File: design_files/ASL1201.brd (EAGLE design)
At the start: 12.5 x 18.5 mm, 3 parts, among them J1 LPPB051NGCN-RC, J2 S2B-PH-SM4

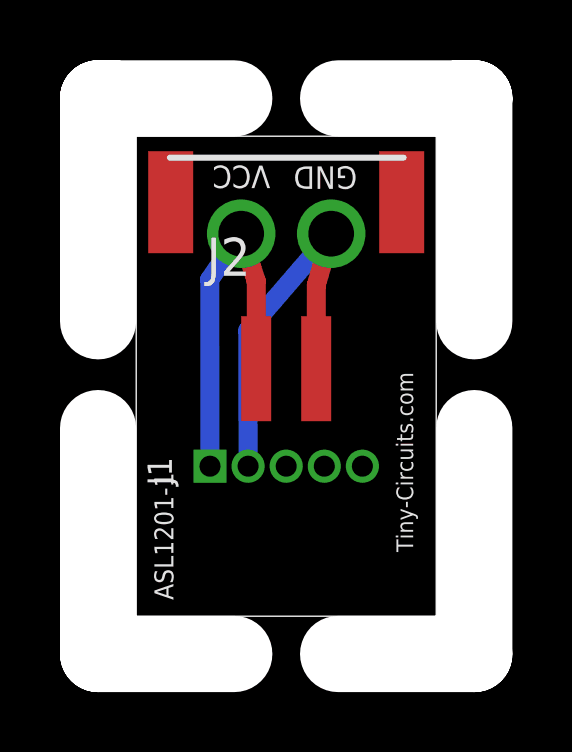
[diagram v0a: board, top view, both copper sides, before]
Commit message: update format
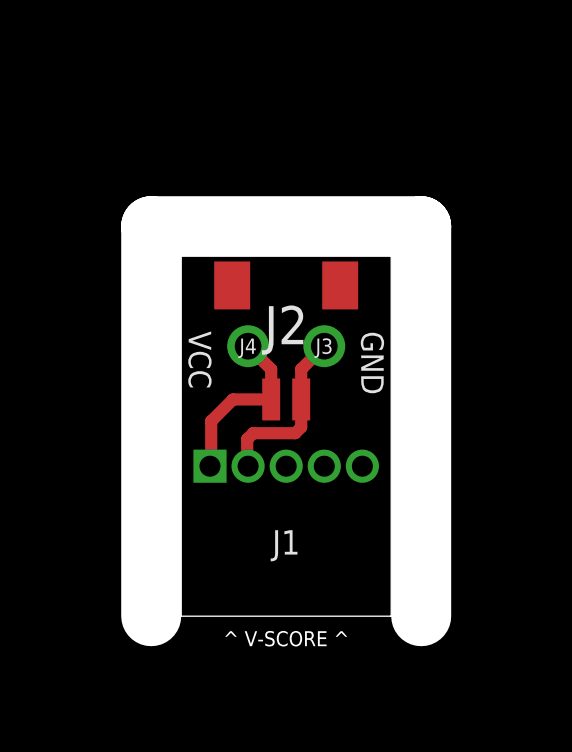
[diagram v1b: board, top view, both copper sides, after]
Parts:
- added J3, J4: PIN_1X.1"1, tinycircuits:1X.1"_2
- J2: value S2B-PH-SM4 -> SM02B-SRSS-TB(LF)(SN); device tinycircuits:JST_PH_2 -> tinycircuits:JST_SH_2X1
- moved J2 1.30 mm to (20.0, 22.7), turned to 180 degrees
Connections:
- removed net GND: J1.2, J2.1
- removed net VCC: J1.1, J2.2
- new net N$1: J1.1, J2.2, J4.1
- new net N$2: J1.2, J2.1, J3.1
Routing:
- net GND: track 13.4 -> 0.00 mm, vias 1 -> 0
- net VCC: track 12.7 -> 0.00 mm, vias 1 -> 0
- net N$1: track 0.00 -> 5.91 mm
- net N$2: track 0.00 -> 5.90 mm
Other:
- board size 12.5 x 18.5 mm -> 9 x 13 mm
- board text added: "2"
- board text added: "ASL1201-2"
- board text added: "TinyCircuits"
- board text added: "^ V-SCORE ^"
- board text removed: "1"
- board text removed: "ASL1201-1"
- board text removed: "Tiny-Circuits.com"
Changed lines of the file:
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@@
 <?xml version="1.0" encoding="utf-8"?>
 <!DOCTYPE eagle SYSTEM "eagle.dtd">
-<eagle version="6.2">
+<eagle version="6.3">
 <drawing>
 <settings>
@@
 <setting verticaltext="up"/>
 </settings>
-<grid distance="1" unitdist="mil" unit="mil" style="lines" multiple="1" display="yes" altdistance="0.025" altunitdist="inch" altunit="inch"/>
+<grid distance="0.5" unitdist="mm" unit="mm" style="lines" multiple="1" display="yes" altdistance="0.025" altunitdist="inch" altunit="inch"/>
 <layers>
 <layer number="1" name="Top" color="4" fill="1" visible="yes" active="yes"/>
@@
 <layer number="108" name="Dimension_circle" color="7" fill="1" visible="yes" active="yes"/>
 <layer number="109" name="Dimension_normal" color="7" fill="1" visible="yes" active="yes"/>
+<layer number="110" name="fp0" color="7" fill="1" visible="yes" active="yes"/>
 <layer number="111" name="tGTest" color="4" fill="1" visible="no" active="no"/>
 <layer number="112" name="bGTest" color="1" fill="1" visible="no" active="no"/>
@@
 <layer number="220" name="220bmp" color="7" fill="1" visible="yes" active="yes"/>
 <layer number="221" name="221bmp" color="7" fill="1" visible="yes" active="yes"/>
+<layer number="222" name="222bmp" color="7" fill="1" visible="yes" active="yes"/>
 <layer number="223" name="223bmp" color="7" fill="1" visible="yes" active="yes"/>
 <layer number="224" name="224bmp" color="7" fill="1" visible="yes" active="yes"/>
+<layer number="248" name="Housing" color="7" fill="1" visible="yes" active="yes"/>
+<layer number="249" name="Edge" color="7" fill="1" visible="yes" active="yes"/>
 <layer number="250" name="Descript" color="7" fill="1" visible="yes" active="yes"/>
 <layer number="251" name="SMDround" color="7" fill="1" visible="yes" active="yes"/>
@@
 <board>
 <plain>
-<text x="16.2406" y="13.54354375" size="0.635" layer="21" rot="R90">ASL1201-1</text>
+<text x="22.45645625" y="15.7406" size="0.635" layer="22" rot="MR0">ASL1201-2</text>
 <text x="39.878" y="36.655996875" size="0.635" layer="48" ratio="10">NOTES:</text>
 <text x="39.878" y="34.115996875" size="0.4572" layer="48" ratio="10">2.  ALL DIMENSIONS ARE GIVEN IN INCHES.</text>
@@
 <wire x1="69.85" y1="50.8" x2="0" y2="50.8" width="0.127" layer="48"/>
 <wire x1="0" y1="50.8" x2="0" y2="0" width="0.127" layer="48"/>
-<dimension x1="15" y1="29" x2="25" y2="29" x3="20.27340625" y3="32.365109375" layer="48"/>
+<dimension x1="16.5" y1="25" x2="23.5" y2="25" x3="20" y3="28.365109375" layer="48"/>
 <text x="48.111025" y="4.365003125" size="0.889" layer="48">TinyLily Power Adapter Bd</text>
 <text x="44.986825" y="1.7714" size="0.889" layer="48">AS-PCB-ASL1201</text>
-<text x="67.3810375" y="1.6952" size="0.889" layer="48">1</text>
-<text x="23.674046875" y="21.1349125" size="0.5588" layer="21" rot="R270">Tiny-Circuits.com</text>
-<wire x1="15" y1="13" x2="25" y2="13" width="0.0254" layer="20"/>
-<wire x1="25" y1="13" x2="25" y2="29" width="0.0254" layer="20"/>
-<wire x1="25" y1="29" x2="15" y2="29" width="0.0254" layer="20"/>
-<wire x1="15" y1="29" x2="15" y2="13" width="0.0254" layer="20"/>
-<dimension x1="15.5" y1="29" x2="15.5" y2="13" x3="14" y3="21" layer="48"/>
-<wire x1="14.23" y1="30.27" x2="13.73" y2="30.26" width="2.54" layer="46"/>
-<wire x1="13.73" y1="30.26" x2="13.73" y2="22.83" width="2.54" layer="46"/>
-<wire x1="13.73" y1="19.27" x2="13.73" y2="11.74" width="2.54" layer="46"/>
-<wire x1="26.27" y1="22.83" x2="26.27" y2="30.26" width="2.54" layer="46"/>
-<wire x1="26.27" y1="30.26" x2="25.77" y2="30.27" width="2.54" layer="46"/>
-<wire x1="26.27" y1="11.74" x2="26.27" y2="19.27" width="2.54" layer="46"/>
-<wire x1="21.73" y1="30.26" x2="26.27" y2="30.26" width="2.54" layer="46"/>
-<wire x1="13.73" y1="30.26" x2="18.27" y2="30.26" width="2.54" layer="46"/>
-<wire x1="18.27" y1="11.74" x2="13.73" y2="11.74" width="2.54" layer="46"/>
-<wire x1="26.27" y1="11.74" x2="21.73" y2="11.74" width="2.54" layer="46"/>
-<wire x1="15" y1="29" x2="15" y2="13" width="0.0254" layer="109"/>
-<wire x1="25" y1="29" x2="25" y2="13" width="0.0254" layer="109"/>
-<wire x1="25" y1="29" x2="15" y2="29" width="0.0254" layer="109"/>
-<wire x1="25" y1="13" x2="15" y2="13" width="0.0254" layer="109"/>
+<text x="67.3810375" y="1.6952" size="0.889" layer="48">2</text>
+<text x="17.3650875" y="20.174046875" size="0.5588" layer="22" rot="MR180">TinyCircuits</text>
+<wire x1="16.5" y1="13" x2="23.5" y2="13" width="0.0254" layer="20"/>
+<wire x1="23.5" y1="13" x2="23.5" y2="25" width="0.0254" layer="20"/>
+<wire x1="23.5" y1="25" x2="16.5" y2="25" width="0.0254" layer="20"/>
+<wire x1="16.5" y1="25" x2="16.5" y2="13" width="0.0254" layer="20"/>
+<dimension x1="15.5" y1="25" x2="15.5" y2="13" x3="15.5" y3="19" layer="48"/>
+<wire x1="15.5" y1="26" x2="15.5" y2="13" width="2" layer="46"/>
+<wire x1="24.5" y1="13" x2="24.5" y2="26" width="2" layer="46"/>
+<wire x1="15.5" y1="26" x2="24.5" y2="26" width="2" layer="46"/>
+<wire x1="16.5" y1="25" x2="16.5" y2="13" width="0.0254" layer="109"/>
+<wire x1="23.5" y1="25" x2="23.5" y2="13" width="0.0254" layer="109"/>
+<wire x1="23.5" y1="25" x2="16.5" y2="25" width="0.0254" layer="109"/>
+<wire x1="23.5" y1="13" x2="16.5" y2="13" width="0.0254" layer="109"/>
 <text x="40.0812" y="14.227796875" size="0.4572" layer="48" ratio="10">Released under the Creative Commons Attribution Share-Alike 3.0 License</text>
 <text x="40.0812" y="13.465796875" size="0.4572" layer="48" ratio="10">http://creativecommons.org/licenses/by-sa/3.0</text>
 <text x="40.0812" y="12.195796875" size="0.4572" layer="48" ratio="10">Original Arduino Uno Design by Team Arduino</text>
 <text x="40.0812" y="11.433796875" size="0.4572" layer="48" ratio="10">LilyPad Arduino Design by Leah Buechley and Sparkfun Electronics</text>
-<text x="19.46985625" y="28.0196" size="0.75" layer="21" rot="SR180">VCC</text>
-<text x="22.36545625" y="27.9942" size="0.75" layer="21" rot="SR180">GND</text>
+<text x="17.5" y="22.5" size="0.75" layer="21" rot="SR270" align="top-left">VCC</text>
+<text x="22.5" y="22.5" size="0.75" layer="21" rot="SR270">GND</text>
 <text x="40.0812" y="10.722596875" size="0.4572" layer="48" ratio="10">TinyDuino, TinyLily and TinyShield Designs by TinyCircuits</text>
+<text x="20" y="12" size="0.5" layer="20" align="bottom-center">^ V-SCORE ^</text>
 </plain>
 <attributes>
@@
 </class>
 </classes>
-<designrules>
+<designrules name="default">
 <description language="de">&lt;b&gt;EAGLE Design Rules&lt;/b&gt;
 &lt;p&gt;
@@
 <attribute name="VALUE" value="LPPB051NGCN-RC" x="20" y="18" size="1.778" layer="27" rot="R90" display="off"/>
 </element>
-<element name="J2" library="tinycircuits" package="JST_PH_2" value="S2B-PH-SM4" x="20" y="24">
-<attribute name="PARTNO" value="AS-ITM-00043" x="20" y="24" size="1.778" layer="27" display="off"/>
-<attribute name="VALUE" value="S2B-PH-SM4" x="20" y="24" size="1.778" layer="27" display="off"/>
+<element name="J2" library="tinycircuits" package="JST_SH_2X1" value="SM02B-SRSS-TB(LF)(SN)" x="20" y="22.7" rot="R180">
+<attribute name="PARTNO" value="AS-ITM-00231" x="20" y="22.7" size="1.778" layer="27" rot="R180" display="off"/>
+<attribute name="VALUE" value="SM02B-SRSS-TB(LF)(SN)" x="20" y="22.7" size="1.778" layer="27" rot="R180" display="off"/>
+</element>
+<element name="J4" library="tinycircuits" package="1X.1&quot;_2" value="PIN_1X.1&quot;1" x="18.73" y="22"/>
+<element name="J3" library="tinycircuits" package="1X.1&quot;_2" value="PIN_1X.1&quot;1" x="21.27" y="22">
+<attribute name="DATABASE" value="./../../../../../Components/TinyCircuits_Part_Database.txt" x="21.27" y="22" size="1.778" layer="27" display="off"/>
 </element>
 </elements>
 <signals>
-<signal name="VCC">
-<contactref element="J1" pad="1"/>
-<contactref element="J2" pad="2"/>
-<via x="18.5" y="25.75" extent="1-16" drill="1.524"/>
-<wire x1="19" y1="21.25" x2="18.9992" y2="24.1742" width="0.635" layer="1"/>
-<wire x1="18.9992" y1="24.1742" x2="18.5" y2="25.75" width="0.635" layer="1"/>
-<wire x1="17.46" y1="18" x2="17.4498" y2="24.225" width="0.635" layer="16"/>
-<wire x1="17.4498" y1="24.225" x2="18.5" y2="25.75" width="0.635" layer="16"/>
-</signal>
 <signal name="N$13">
 </signal>
 <signal name="OSCO">
 </signal>
-<signal name="GND">
+<signal name="N$1">
+<contactref element="J2" pad="2"/>
+<contactref element="J4" pad="1"/>
+<contactref element="J1" pad="1"/>
+<wire x1="18.73" y1="22" x2="19.5" y2="21.23" width="0.4064" layer="1"/>
+<wire x1="19.5" y1="21.23" x2="19.5" y2="20.225" width="0.4064" layer="1"/>
+<wire x1="19.5" y1="20.225" x2="18.225" y2="20.225" width="0.4064" layer="1"/>
+<wire x1="18.225" y1="20.225" x2="17.5" y2="19.5" width="0.4064" layer="1"/>
+<wire x1="17.5" y1="19.5" x2="17.5" y2="18.04" width="0.4064" layer="1"/>
+<wire x1="17.5" y1="18.04" x2="17.46" y2="18" width="0.4064" layer="1"/>
+</signal>
+<signal name="N$2">
 <contactref element="J1" pad="2"/>
 <contactref element="J2" pad="1"/>
-<via x="21.5" y="25.75" extent="1-16" drill="1.524"/>
-<wire x1="21" y1="21.25" x2="21.0058" y2="24.0472" width="0.635" layer="1"/>
-<wire x1="21.0058" y1="24.0472" x2="21.5" y2="25.75" width="0.635" layer="1"/>
-<wire x1="18.73" y1="18" x2="18.7198" y2="22.5232" width="0.635" layer="16"/>
-<wire x1="18.7198" y1="22.5232" x2="21.5" y2="25.75" width="0.635" layer="16"/>
+<contactref element="J3" pad="1"/>
+<wire x1="21.27" y1="22" x2="20.5" y2="21.23" width="0.4064" layer="1"/>
+<wire x1="20.5" y1="21.23" x2="20.5" y2="20.225" width="0.4064" layer="1"/>
+<wire x1="20.5" y1="20.225" x2="20.5" y2="19.3" width="0.4064" layer="1"/>
+<wire x1="20.5" y1="19.3" x2="20.3" y2="19.1" width="0.4064" layer="1"/>
+<wire x1="20.3" y1="19.1" x2="18.9" y2="19.1" width="0.4064" layer="1"/>
+<wire x1="18.9" y1="19.1" x2="18.7" y2="18.9" width="0.4064" layer="1"/>
+<wire x1="18.7" y1="18.9" x2="18.7" y2="18.03" width="0.4064" layer="1"/>
+<wire x1="18.7" y1="18.03" x2="18.73" y2="18" width="0.4064" layer="1"/>
 </signal>
 </signals>
